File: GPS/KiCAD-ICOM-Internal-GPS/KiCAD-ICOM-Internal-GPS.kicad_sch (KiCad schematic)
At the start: 4 parts, among them J1 ICOM-J1, J2 U.FL-R-SMT-1_10_, U1 MAX-M10M-00B

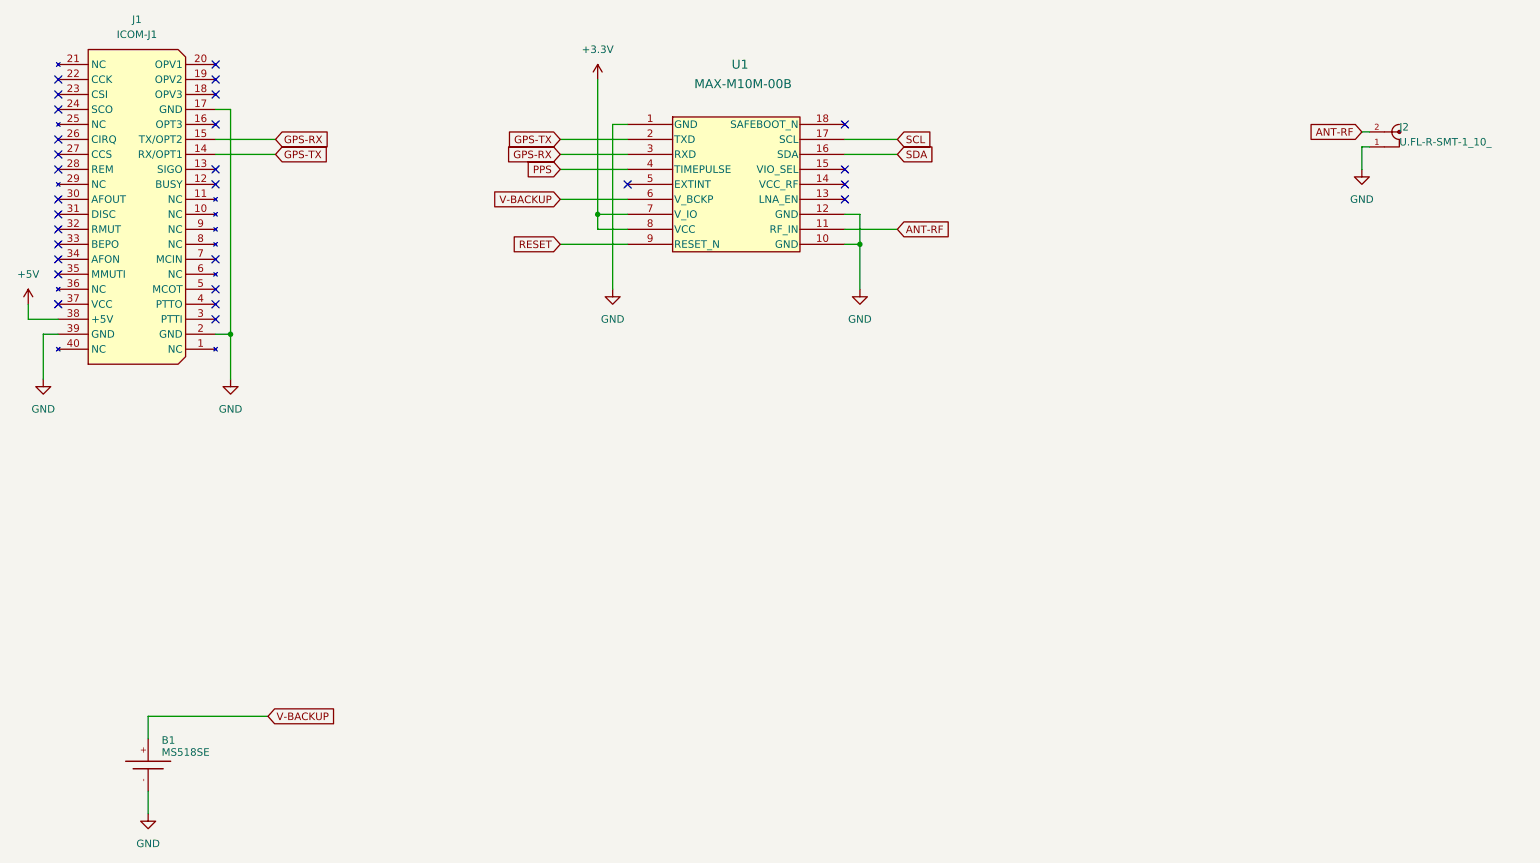
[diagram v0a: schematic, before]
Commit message: updated schematic and pcb
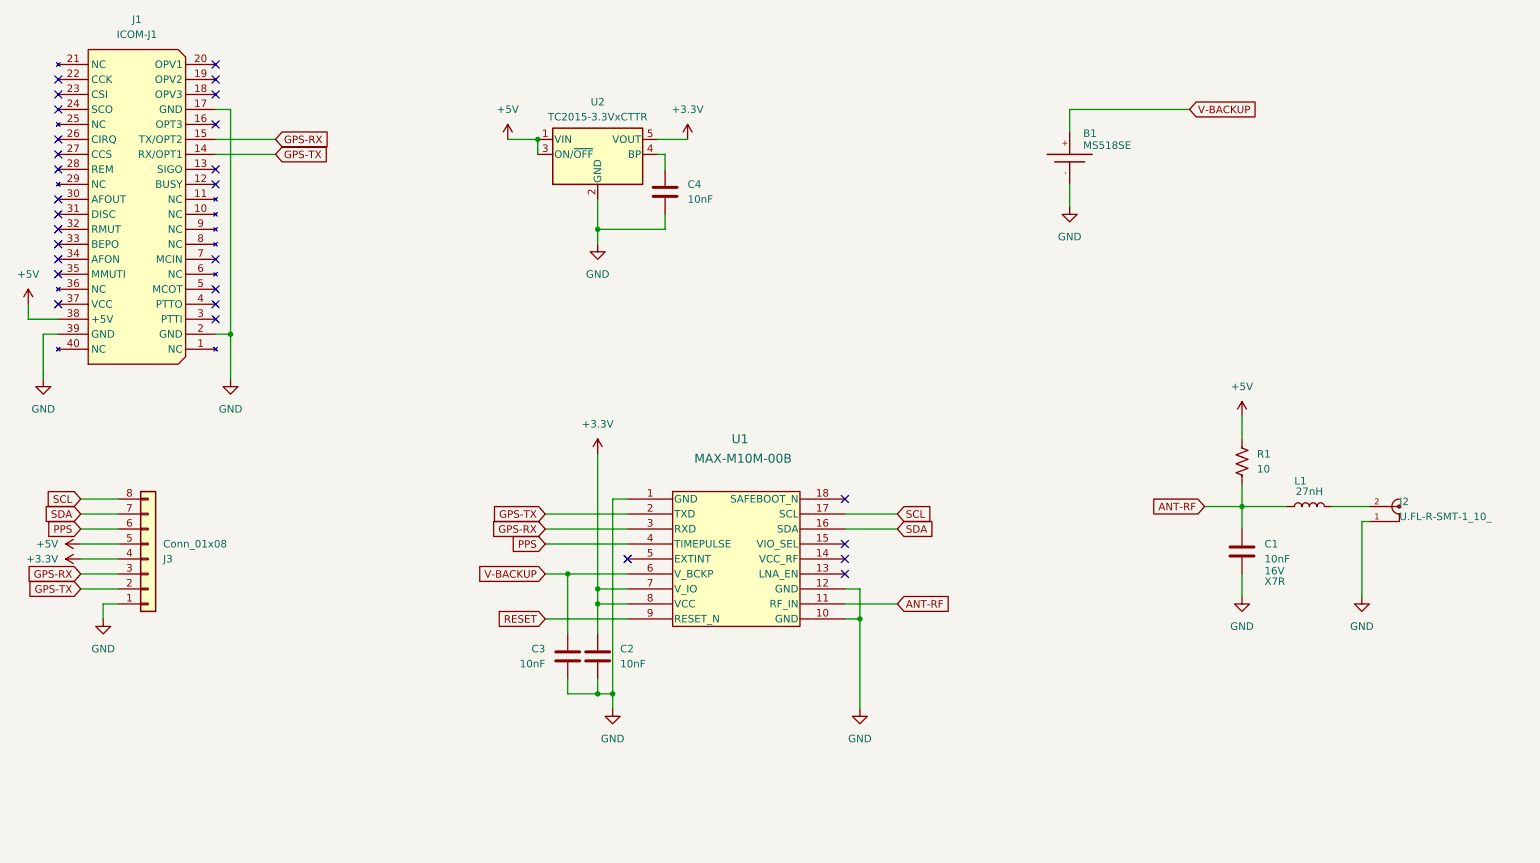
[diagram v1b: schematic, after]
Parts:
- added C1, C2, C3, C4: 10nF, Capacitor_SMD:C_0603_1608Metric, symbol Device:C
- added J3: Conn_01x08, Connector_PinSocket_2.54mm:PinSocket_1x08_P2.54mm_Vertical, symbol Connector_Generic:Conn_01x08
- added L1: 27nH, Inductor_SMD:L_0402_1005Metric, symbol Device:L
- added R1: 10, Resistor_SMD:R_0603_1608Metric, symbol Device:R_US
- added U2: TC2015-3.3VxCTTR, Package_TO_SOT_SMD:SOT-23-5, symbol Regulator_Linear:TC2015-3.3VxCTTR
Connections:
- net +3.3V: now also C2.1, J3.4 (Pin_4), U2.5 (VOUT)
- net +5V: now also J3.5 (Pin_5), R1.1, U2.1 (VIN), U2.3 (ON/~{OFF})
- net ANT-RF: now also C1.1, L1.1, R1.2; no longer J2.2
- net GND: now also C1.2, C2.2, C3.2, C4.2, J3.1 (Pin_1), U2.2 (GND)
- net GPS-RX: now also J3.3 (Pin_3)
- net GPS-TX: now also J3.2 (Pin_2)
- net PPS: now also J3.6 (Pin_6)
- net SCL: now also J3.8 (Pin_8)
- net SDA: now also J3.7 (Pin_7)
- net V-BACKUP: now also C3.1
- new net: J2.2, L1.2
- new net: C4.1, U2.4 (BP)
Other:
- moved on the sheet: B1, J2, U1
